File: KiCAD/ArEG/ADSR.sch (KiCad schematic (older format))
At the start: 34 parts

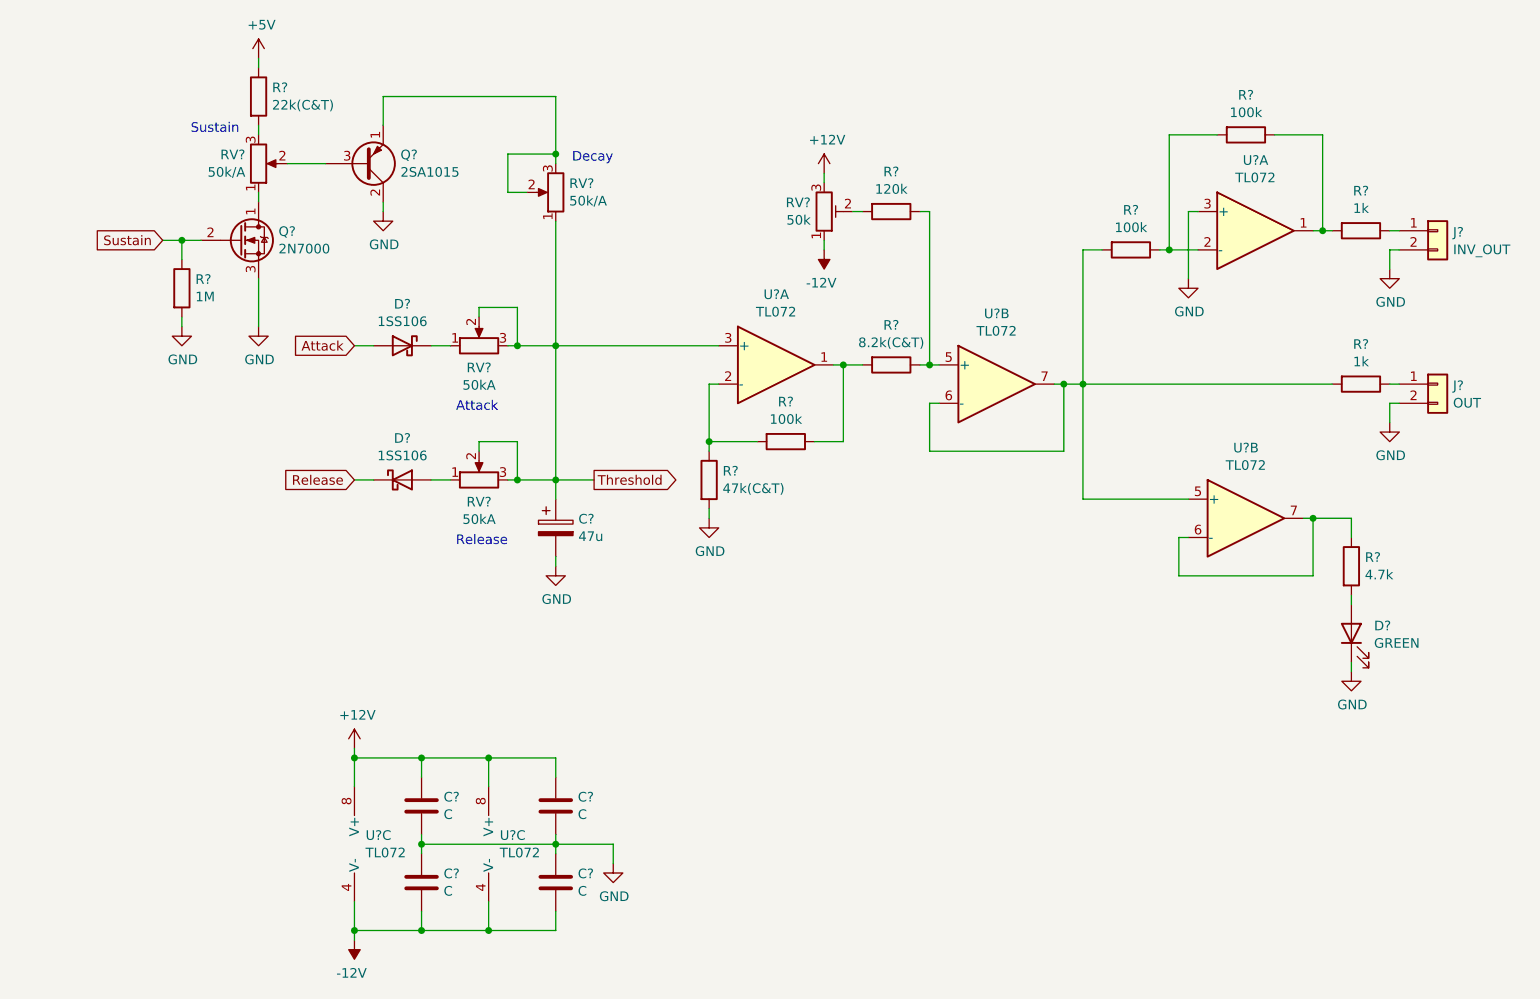
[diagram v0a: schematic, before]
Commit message: 入出力端子をまとめる前
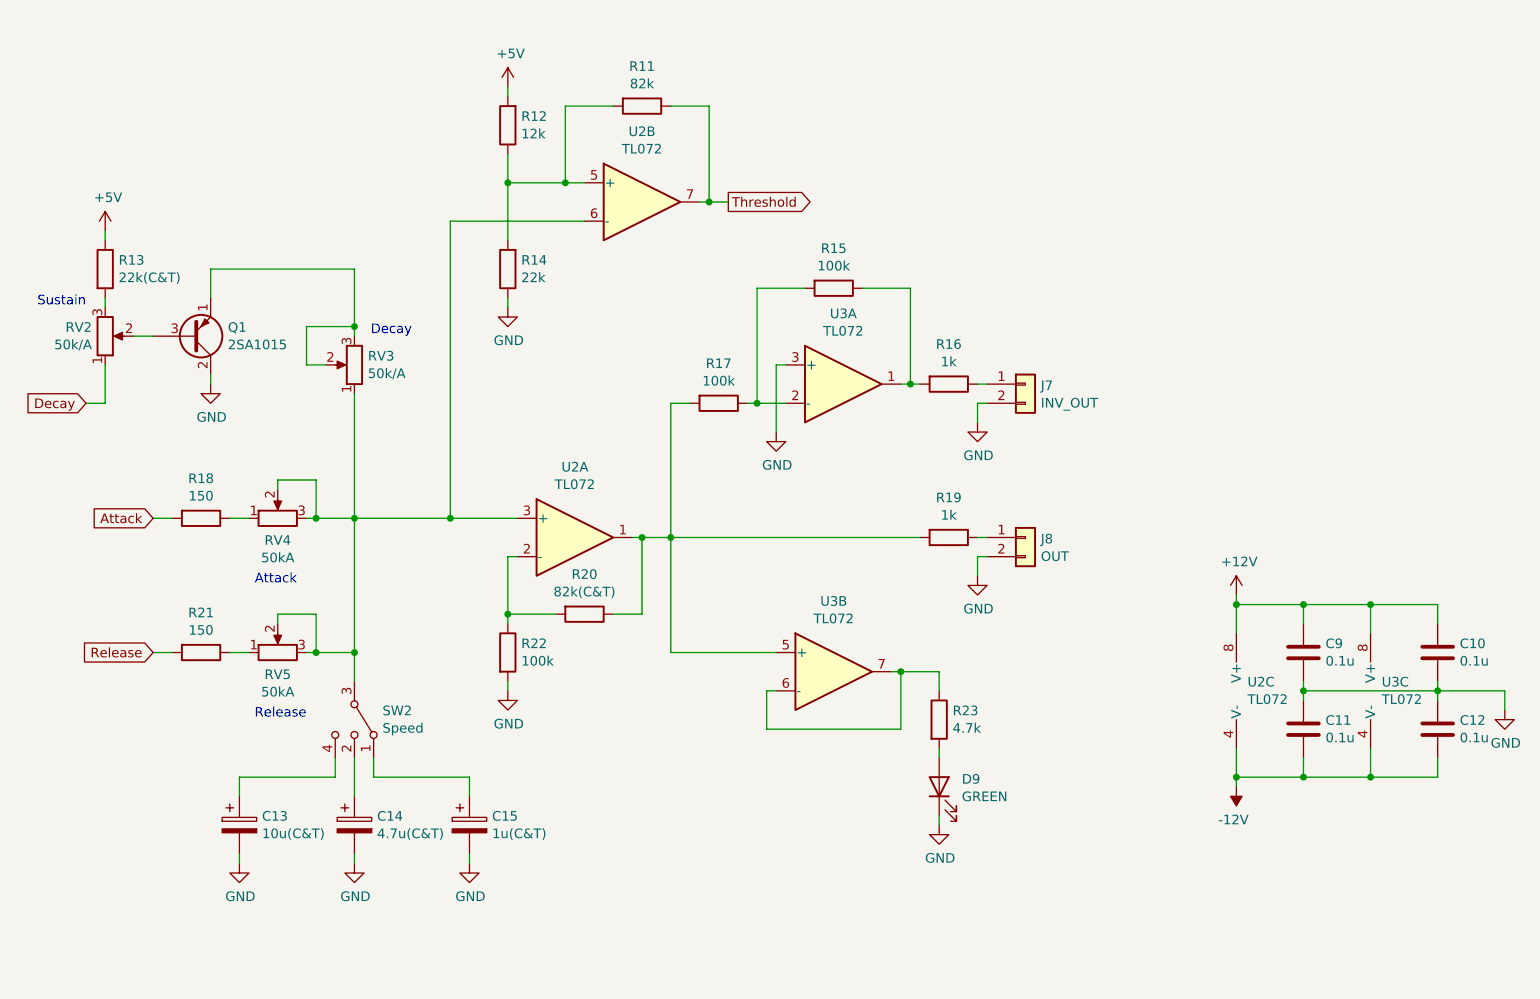
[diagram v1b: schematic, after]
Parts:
- removed D? (x2): 1SS106, symbol Device:D_Schottky
- removed Q?: 2N7000, symbol Device:Q_NMOS_DGS
- removed R?: 1M, symbol Device:R
- removed R?: 8.2k(C&T), symbol Device:R
- removed R?: 120k, symbol Device:R
- removed RV?: 50k, symbol Device:R_POT_TRIM
- removed U?: TL072, symbol Amplifier_Operational:TL072
- added C14: 4.7u(C&T), Capacitor_THT:CP_Radial_D5.0mm_P2.50mm, symbol Device:CP
- added C15: 1u(C&T), Capacitor_THT:CP_Radial_D5.0mm_P2.50mm, symbol Device:CP
- added R11: 82k, Resistor_THT:R_Axial_DIN0207_L6.3mm_D2.5mm_P10.16mm_Horizontal, symbol Device:R
- added R12: 12k, Resistor_THT:R_Axial_DIN0207_L6.3mm_D2.5mm_P10.16mm_Horizontal, symbol Device:R
- added R14: 22k, Resistor_THT:R_Axial_DIN0207_L6.3mm_D2.5mm_P10.16mm_Horizontal, symbol Device:R
- added R18, R21: 150, Resistor_THT:R_Axial_DIN0207_L6.3mm_D2.5mm_P10.16mm_Horizontal, symbol Device:R
- added SW2: Speed, Connector_JST:JST_XH_B4B-XH-A_1x04_P2.50mm_Vertical, symbol Switch:SW_SP3T
- added unit 2 of U2
- C10, C11, C12, C9: renamed from C?; value C -> 0.1u; footprint (none) -> Capacitor_THT:C_Disc_D3.0mm_W1.6mm_P2.50mm
- C13: renamed from C?; value 47u -> 10u(C&T); footprint (none) -> Capacitor_THT:CP_Radial_D5.0mm_P2.50mm
- D9: renamed from D?; footprint (none) -> Connector_JST:JST_XH_B2B-XH-A_1x02_P2.50mm_Vertical
- J7, J8: renamed from J?; footprint (none) -> Connector_JST:JST_XH_B2B-XH-A_1x02_P2.50mm_Vertical
- Q1: renamed from Q?; footprint (none) -> Package_TO_SOT_THT:TO-92_Wide
- R13, R15, R16, R17, R19, R23: renamed from R?; footprint (none) -> Resistor_THT:R_Axial_DIN0207_L6.3mm_D2.5mm_P10.16mm_Horizontal
- R20: renamed from R?; value 100k -> 82k(C&T); footprint (none) -> Resistor_THT:R_Axial_DIN0207_L6.3mm_D2.5mm_P10.16mm_Horizontal
- R22: renamed from R?; value 47k(C&T) -> 100k; footprint (none) -> Resistor_THT:R_Axial_DIN0207_L6.3mm_D2.5mm_P10.16mm_Horizontal
- RV2, RV3, RV4, RV5: renamed from RV?; footprint (none) -> Potentiometer_THT:Potentiometer_Alps_RK09Y11_Single_Horizontal
- U2, U3: renamed from U?; footprint (none) -> Package_DIP:DIP-8_W7.62mm_LongPads
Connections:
- net +5V: now also R12.2
- net Attack: now also R18.2
- net GND: now also C14.2, C15.2, R14.1
- net Release: now also R21.2
- net Threshold: now also R11.1, U2.7; no longer C13.1, RV3.1, RV4.2, RV4.3, RV5.2, RV5.3, U2.3 (+)
- net Decay: now reaches RV2.1
- net at RV4.1: now also R18.1
- net at RV5.1: now also R21.1
- net at R17.2, R19.2, U3.5 (+): now also R20.1, U2.1
- new net: RV3.1, RV4.2, RV4.3, RV5.2, RV5.3, SW2.3, U2.3 (+), U2.6 (-)
- new net: C13.1, SW2.4
- new net: C15.1, SW2.1
- new net: C14.1, SW2.2
- new net: R11.2, R12.1, R14.2, U2.5 (+)
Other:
- moved on the sheet: C10, C11, C12, C13, C9, D9, J7, J8, Q1, R13, R15, R16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

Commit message: Panel design
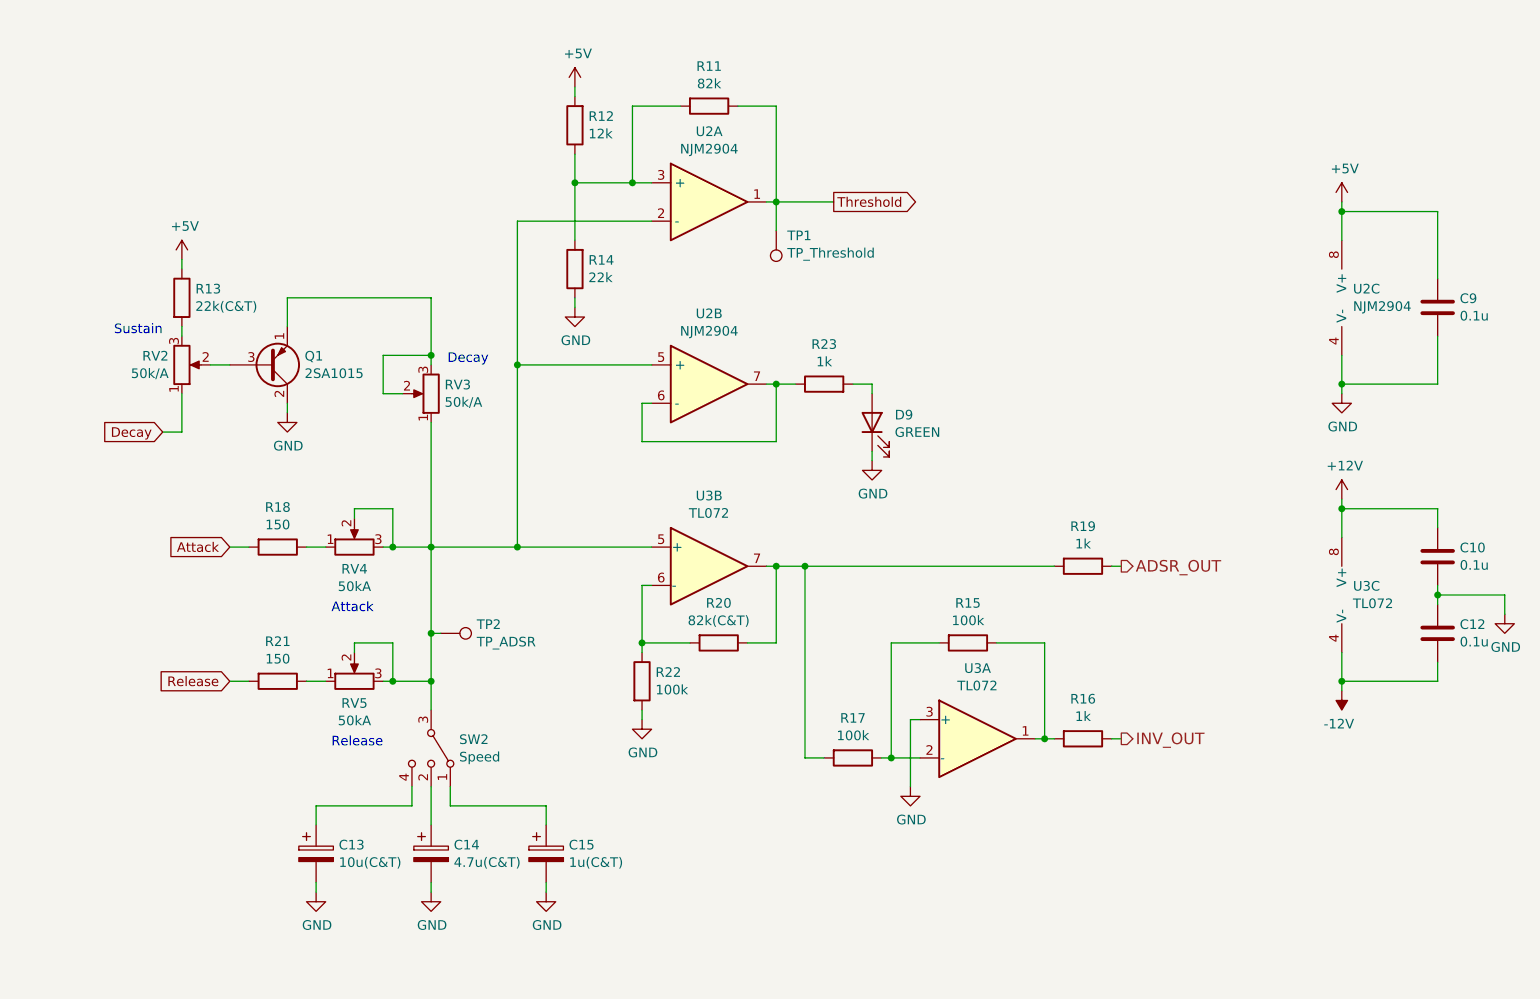
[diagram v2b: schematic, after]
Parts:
- removed C11: 0.1u, Capacitor_THT:C_Disc_D3.0mm_W1.6mm_P2.50mm, symbol Device:C
- removed J7: INV_OUT, Connector_JST:JST_XH_B2B-XH-A_1x02_P2.50mm_Vertical, symbol Connector_Generic:Conn_01x02
- removed J8: OUT, Connector_JST:JST_XH_B2B-XH-A_1x02_P2.50mm_Vertical, symbol Connector_Generic:Conn_01x02
- removed unit 3 of U2
- removed unit 2 of U2
- removed unit 2 of U3
- added TP1: TP_Threshold, TestPoint:TestPoint_Pad_D1.0mm, symbol Connector:TestPoint
- added TP2: TP_ADSR, TestPoint:TestPoint_Pad_D1.0mm, symbol Connector:TestPoint
- added U2: NJM2904, Package_DIP:DIP-8_W7.62mm_Socket_LongPads, symbol Device:Opamp_Dual_Generic
- R23: value 4.7k -> 1k
- U3: footprint Package_DIP:DIP-8_W7.62mm_LongPads -> Package_DIP:DIP-8_W7.62mm_Socket_LongPads
- U3: renamed from U2; footprint Package_DIP:DIP-8_W7.62mm_LongPads -> Package_DIP:DIP-8_W7.62mm_Socket_LongPads
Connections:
- net +12V: no longer C9.1
- net +5V: now also C9.1, U2.8 (V+)
- net GND: now also U2.4 (V-)
- net Threshold: now also TP1.1, U2.1
- net at RV3.1, RV4.2, RV4.3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: now also U3.5 (+), TP2.1, U2.2 (-), U2.5 (+); no longer U3.3 (+)
- net INV_OUT: now reaches R16.1
- net ADSR_OUT: now reaches R19.1
- net at R17.2, R19.2, R20.1: now also U3.7; no longer U3.1
- net at R20.2, R22.1: now also U3.6 (-); no longer U3.2 (-)
- net at R23.1: now also U2.6 (-), U2.7
- net at R11.2, R12.1, R14.2: now also U2.3 (+)
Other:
- moved on the sheet: C10, C12, C13, C14, C15, C9, D9, Q1, R11, R12, R13, R14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
